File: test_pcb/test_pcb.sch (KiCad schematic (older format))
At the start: 66 parts, among them K0 KEYSW, K1 KEYSW, K10 KEYSW, K12 KEYSW, K13 KEYSW, K14 KEYSW, K15 KEYSW, K16 KEYSW, K17 KEYSW, K18 KEYSW, K2 KEYSW, K20 KEYSW, K21 KEYSW, K22 KEYSW, K3 KEYSW, K4 KEYSW, K5 KEYSW, K6 KEYSW, K7 KEYSW, K8 KEYSW, K9 KEYSW, P0 CONN_01X08, U0 Teensy3.2, U1 STP16CP05

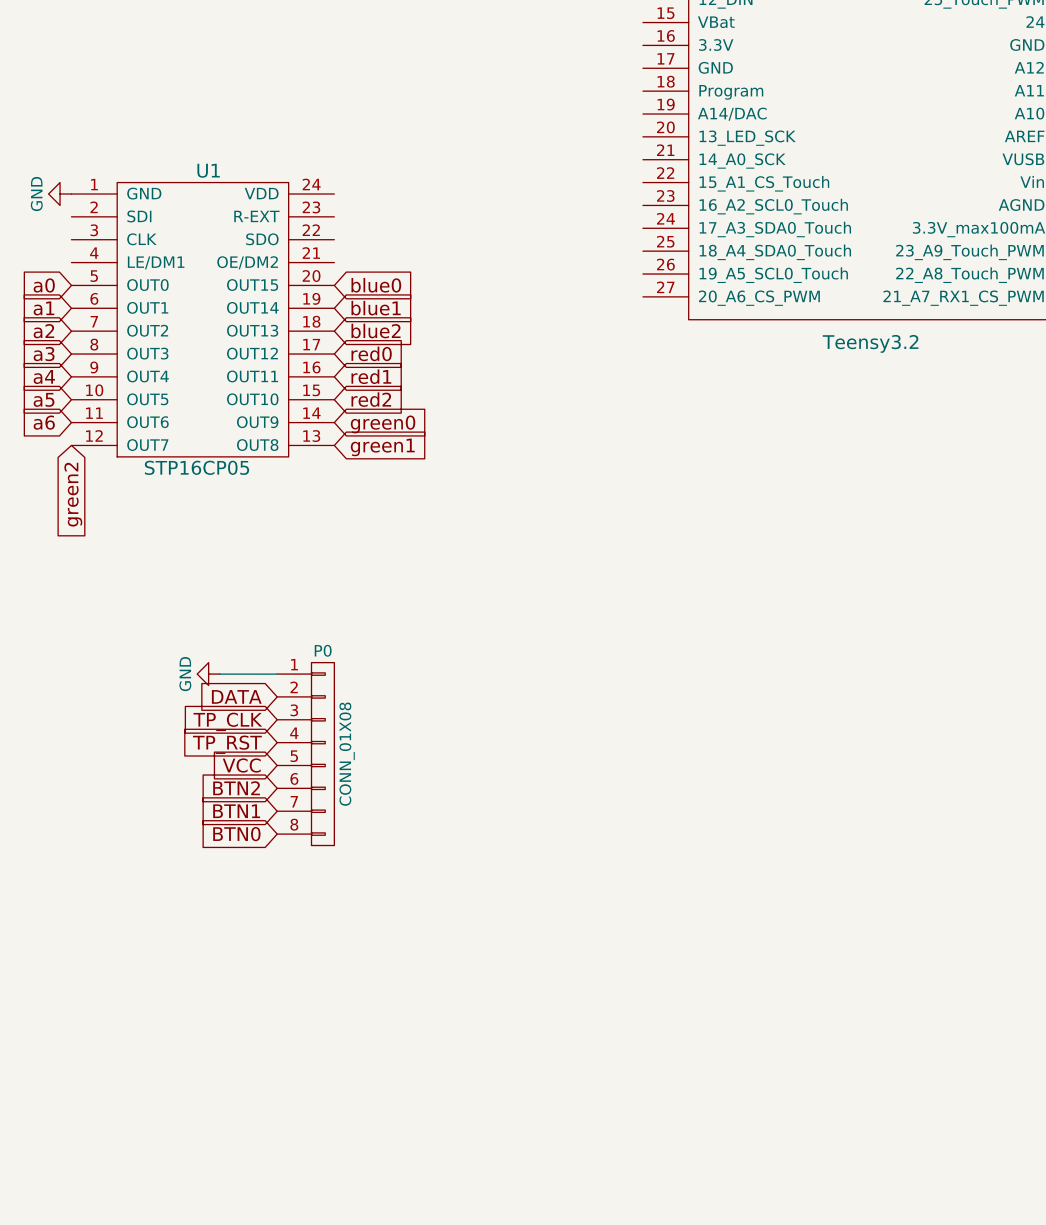
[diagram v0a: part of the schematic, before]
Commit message: updates?
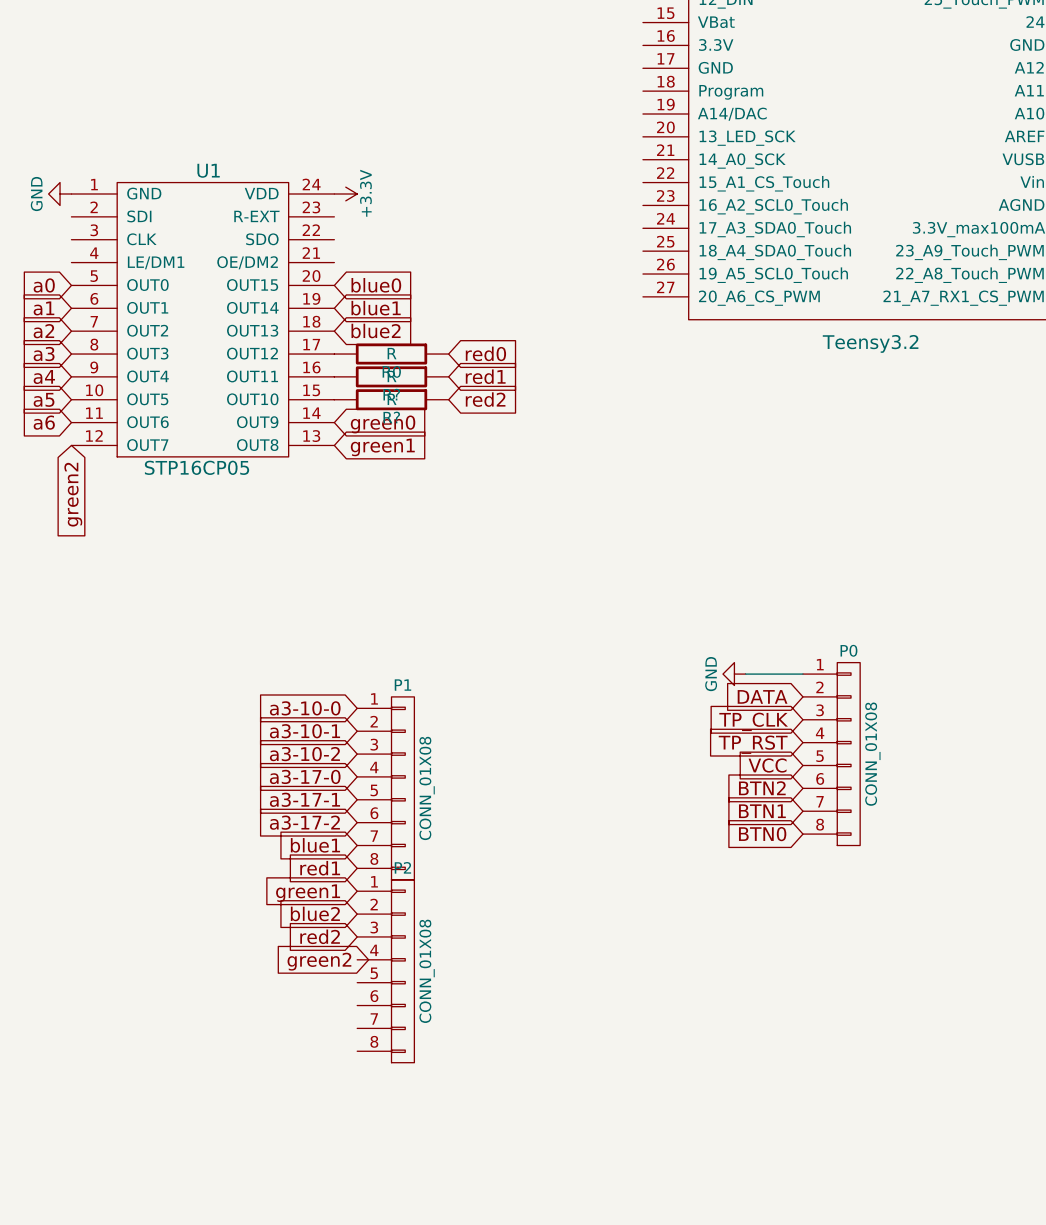
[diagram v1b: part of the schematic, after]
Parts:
- added P1, P2: CONN_01X08, Connectors_Molex:Molex_PicoBlade_53261-0871_08x1.25mm_Angled, symbol CONN_01X08
- added R0, R? (x2): R, symbol R
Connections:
- net labels added: +3.3V
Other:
- moved on the sheet: P0
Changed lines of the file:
@@
 L CONN_01X08 P0
 U 1 1 5897F60A
-P 7600 5300
-F 0 "P0" H 7600 5750 50  0000 C CNN
-F 1 "CONN_01X08" V 7700 5300 50  0000 C CNN
-F 2 "Connectors_Molex:Molex_PicoBlade_53261-0871_08x1.25mm_Angled" H 7600 5300 50  0001 C CNN
-F 3 "" H 7600 5300 50  0000 C CNN
-	1    7600 5300
-	1    0    0    -1
-$EndComp
-Text GLabel 7400 5650 0    60   Input ~ 0
+P 9900 5300
+F 0 "P0" H 9900 5750 50  0000 C CNN
+F 1 "CONN_01X08" V 10000 5300 50  0000 C CNN
+F 2 "Connectors_Molex:Molex_PicoBlade_53261-0871_08x1.25mm_Angled" H 9900 5300 50  0001 C CNN
+F 3 "" H 9900 5300 50  0000 C CNN
+	1    9900 5300
+	1    0    0    -1
+$EndComp
+Text GLabel 9700 5650 0    60   Input ~ 0
 BTN0
-Text GLabel 7400 5550 0    60   Input ~ 0
+Text GLabel 9700 5550 0    60   Input ~ 0
 BTN1
-Text GLabel 7400 5450 0    60   Input ~ 0
+Text GLabel 9700 5450 0    60   Input ~ 0
 BTN2
-Text GLabel 7400 5350 0    60   Input ~ 0
+Text GLabel 9700 5350 0    60   Input ~ 0
 VCC
-Text GLabel 7400 5050 0    60   Input ~ 0
+Text GLabel 9700 5050 0    60   Input ~ 0
 DATA
-Text GLabel 7400 5250 0    60   Input ~ 0
+Text GLabel 9700 5250 0    60   Input ~ 0
 TP_RST
-Text GLabel 7400 5150 0    60   Input ~ 0
+Text GLabel 9700 5150 0    60   Input ~ 0
 TP_CLK
 $Comp
@@
 Text GLabel 7650 3250 2    60   Input ~ 0
 blue0
-Text GLabel 7650 3550 2    60   Input ~ 0
+Text GLabel 8150 3550 2    60   Input ~ 0
 red0
 Text GLabel 7650 3850 2    60   Input ~ 0
@@
 Text GLabel 7650 3350 2    60   Input ~ 0
 blue1
-Text GLabel 7650 3650 2    60   Input ~ 0
+Text GLabel 8150 3650 2    60   Input ~ 0
 red1
 Text GLabel 7650 3950 2    60   Input ~ 0
@@
 Text GLabel 7650 3450 2    60   Input ~ 0
 blue2
-Text GLabel 7650 3750 2    60   Input ~ 0
+Text GLabel 8150 3750 2    60   Input ~ 0
 red2
 Text GLabel 6500 3950 3    60   Input ~ 0
@@
 a3-17-2
 $Comp
-L GND #PWR?
+L GND #PWR01
 U 1 1 58A59EDB
-P 7150 4950
-F 0 "#PWR?" H 7150 4700 50  0001 C CNN
-F 1 "GND" H 7150 4800 50  0000 C CNN
-F 2 "" H 7150 4950 50  0000 C CNN
-F 3 "" H 7150 4950 50  0000 C CNN
-	1    7150 4950
+P 9450 4950
+F 0 "#PWR01" H 9450 4700 50  0001 C CNN
+F 1 "GND" H 9450 4800 50  0000 C CNN
+F 2 "" H 9450 4950 50  0000 C CNN
+F 3 "" H 9450 4950 50  0000 C CNN
+	1    9450 4950
 	0    1    1    0
 $EndComp
 Wire Wire Line
-	7400 4950 7150 4950
-$Comp
-L GND #PWR?
+	9700 4950 9450 4950
+$Comp
+L GND #PWR02
 U 1 1 58A5AE89
 P 6500 2850
-F 0 "#PWR?" H 6500 2600 50  0001 C CNN
+F 0 "#PWR02" H 6500 2600 50  0001 C CNN
 F 1 "GND" H 6500 2700 50  0000 C CNN
 F 2 "" H 6500 2850 50  0000 C CNN
@@
 	0    1    1    0
 $EndComp
+Text GLabel 7750 5100 0    60   Input ~ 0
+a3-10-0
+Text GLabel 7750 5200 0    60   Input ~ 0
+a3-10-1
+Text GLabel 7750 5300 0    60   Input ~ 0
+a3-10-2
+Text GLabel 7750 5400 0    60   Input ~ 0
+a3-17-0
+Text GLabel 7750 5500 0    60   Input ~ 0
+a3-17-1
+Text GLabel 7750 5600 0    60   Input ~ 0
+a3-17-2
+$Comp
+L +3.3V #PWR03
+U 1 1 58A3C033
+P 7650 2850
+F 0 "#PWR03" H 7650 2700 50  0001 C CNN
+F 1 "+3.3V" H 7650 2990 50  0000 C CNN
+F 2 "" H 7650 2850 50  0000 C CNN
+F 3 "" H 7650 2850 50  0000 C CNN
+	1    7650 2850
+	0    1    1    0
+$EndComp
+$Comp
+L R R0
+U 1 1 58A3D228
+P 7900 3550
+F 0 "R0" V 7980 3550 50  0000 C CNN
+F 1 "R" V 7900 3550 50  0000 C CNN
+F 2 "" H 7900 3550 60  0000 C CNN
+F 3 "" H 7900 3550 60  0000 C CNN
+	1    7900 3550
+	0    1    1    0
+$EndComp
+$Comp
+L R R?
+U 1 1 58A3D3E0
+P 7900 3650
+F 0 "R?" V 7980 3650 50  0000 C CNN
+F 1 "R" V 7900 3650 50  0000 C CNN
+F 2 "" H 7900 3650 60  0000 C CNN
+F 3 "" H 7900 3650 60  0000 C CNN
+	1    7900 3650
+	0    1    1    0
+$EndComp
+$Comp
+L R R?
+U 1 1 58A3D4D0
+P 7900 3750
+F 0 "R?" V 7980 3750 50  0000 C CNN
+F 1 "R" V 7900 3750 50  0000 C CNN
+F 2 "" H 7900 3750 60  0000 C CNN
+F 3 "" H 7900 3750 60  0000 C CNN
+	1    7900 3750
+	0    1    1    0
+$EndComp
+$Comp
+L CONN_01X08 P1
+U 1 1 58A3B45B
+P 7950 5450
+F 0 "P1" H 7950 5900 50  0000 C CNN
+F 1 "CONN_01X08" V 8050 5450 50  0000 C CNN
+F 2 "Connectors_Molex:Molex_PicoBlade_53261-0871_08x1.25mm_Angled" H 7950 5450 50  0001 C CNN
+F 3 "" H 7950 5450 50  0000 C CNN
+	1    7950 5450
+	1    0    0    -1
+$EndComp
+$Comp
+L CONN_01X08 P2
+U 1 1 58A3CB40
+P 7950 6250
+F 0 "P2" H 7950 6700 50  0000 C CNN
+F 1 "CONN_01X08" V 8050 6250 50  0000 C CNN
+F 2 "Connectors_Molex:Molex_PicoBlade_53261-0871_08x1.25mm_Angled" H 7950 6250 50  0001 C CNN
+F 3 "" H 7950 6250 50  0000 C CNN
+	1    7950 6250
+	1    0    0    -1
+$EndComp
+Text GLabel 7750 5700 0    60   Input ~ 0
+blue1
+Text GLabel 7750 5800 0    60   Input ~ 0
+red1
+Text GLabel 7750 5900 0    60   Input ~ 0
+green1
+Text GLabel 7750 6000 0    60   Input ~ 0
+blue2
+Text GLabel 7750 6100 0    60   Input ~ 0
+red2
+Text GLabel 7800 6200 0    60   Input ~ 0
+green2
 $EndSCHEMATC
